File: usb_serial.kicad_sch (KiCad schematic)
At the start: 3 parts, among them U5 CP2104-F03-GM

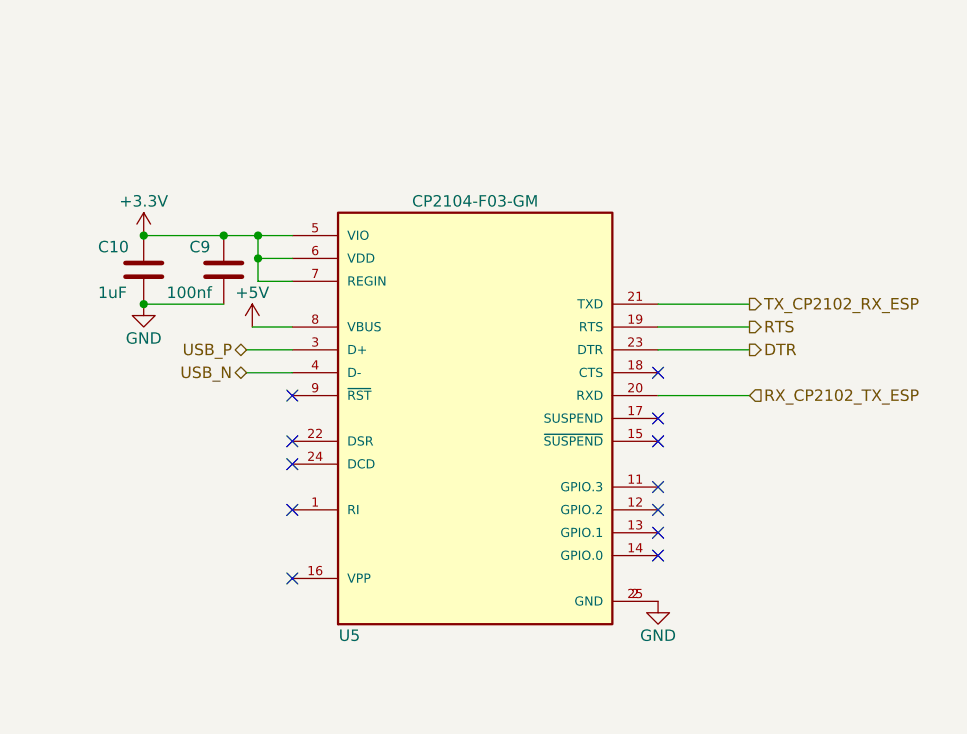
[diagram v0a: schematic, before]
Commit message: laid out stuff
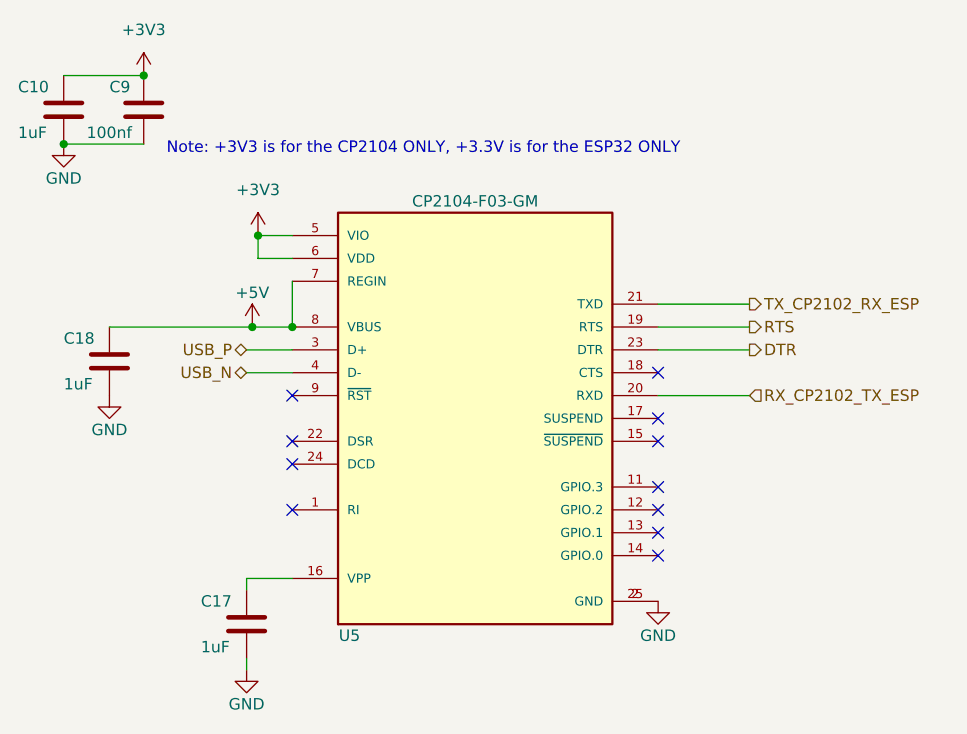
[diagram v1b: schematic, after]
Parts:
- added C17, C18: 1uF, Capacitor_SMD:C_0805_2012Metric_Pad1.18x1.45mm_HandSolder, symbol Device:C
- U5: Availability In Stock -> (none); Check_prices https://www.snapeda.com/parts/CP2104-F03-GM/Silicon+Labs/vi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 -> (none); MANUFACTURER Silicon Labs -> (none); MF Silicon Labs -> (none); MP CP2104-F03-GM -> (none); PARTREV 1.2 -> (none); Package QFN-24 Silicon Labs -> (none); Price None -> (none); Purchase-URL https://www.snapeda.com/api/url_track_click_mouser/?unipart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 -> (none); STANDARD IPC7351B -> (none); SnapEDA_Link https://www.snapeda.com/parts/CP2104-F03-GM/Silicon+Labs/vi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 -> (none)
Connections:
- net +5V: now also U5.7 (REGIN), C18.1
- net GND: now also C17.2, C18.2
- net at U5.16 (VPP): now also C17.1
- net +3.3V renamed +3V3
- net +3V3: no longer U5.7 (REGIN)
- no-connect marks 12 -> 11
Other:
- note added: "Note: +3V3 is for the CP2104 ONLY, +3.3V is for the ESP32 ONLY"
- moved on the sheet: C10, C9

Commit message: neat-ified schematics
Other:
- company: (none) -> The Art and Science of PCB Design
- title: (none) -> RGB LED Driver Demo Board
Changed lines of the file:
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@@
   (paper "USLetter")
   (title_block
+    (title "RGB LED Driver Demo Board")
     (date "2024-01-01")
     (rev "A01")
+    (company "The Art and Science of PCB Design")
   )
   (junction (at 113.665 71.12) (diameter 0) (color 0 0 0 0)
